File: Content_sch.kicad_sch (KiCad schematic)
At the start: 0 parts

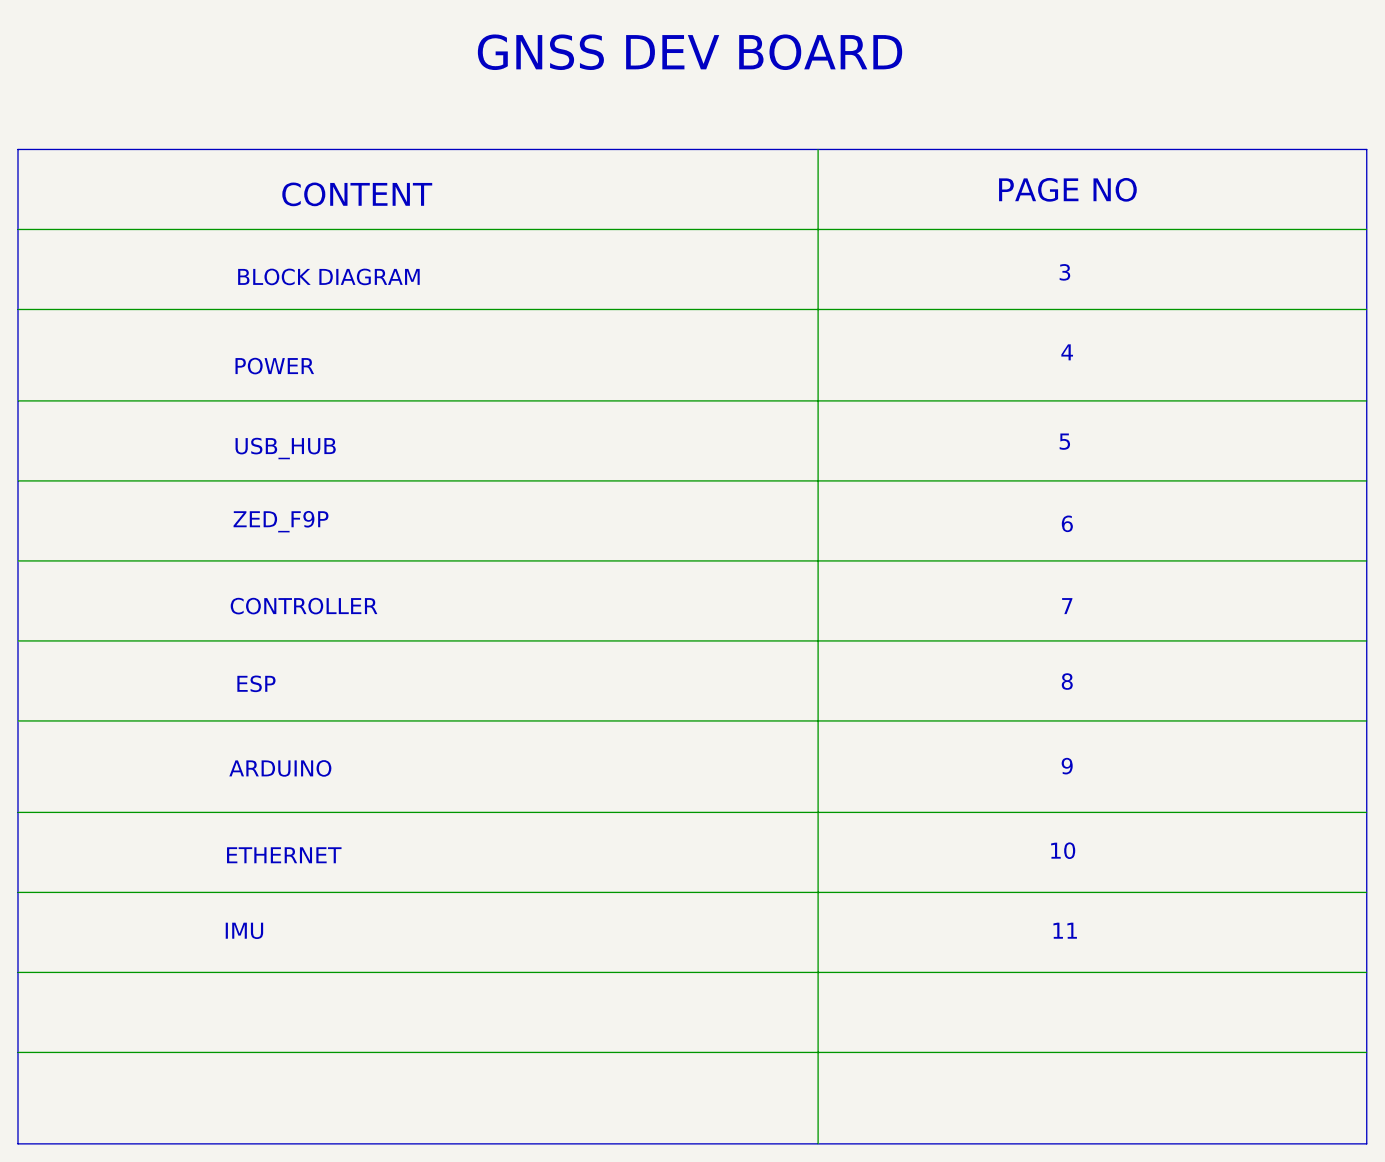
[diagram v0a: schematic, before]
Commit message: changed
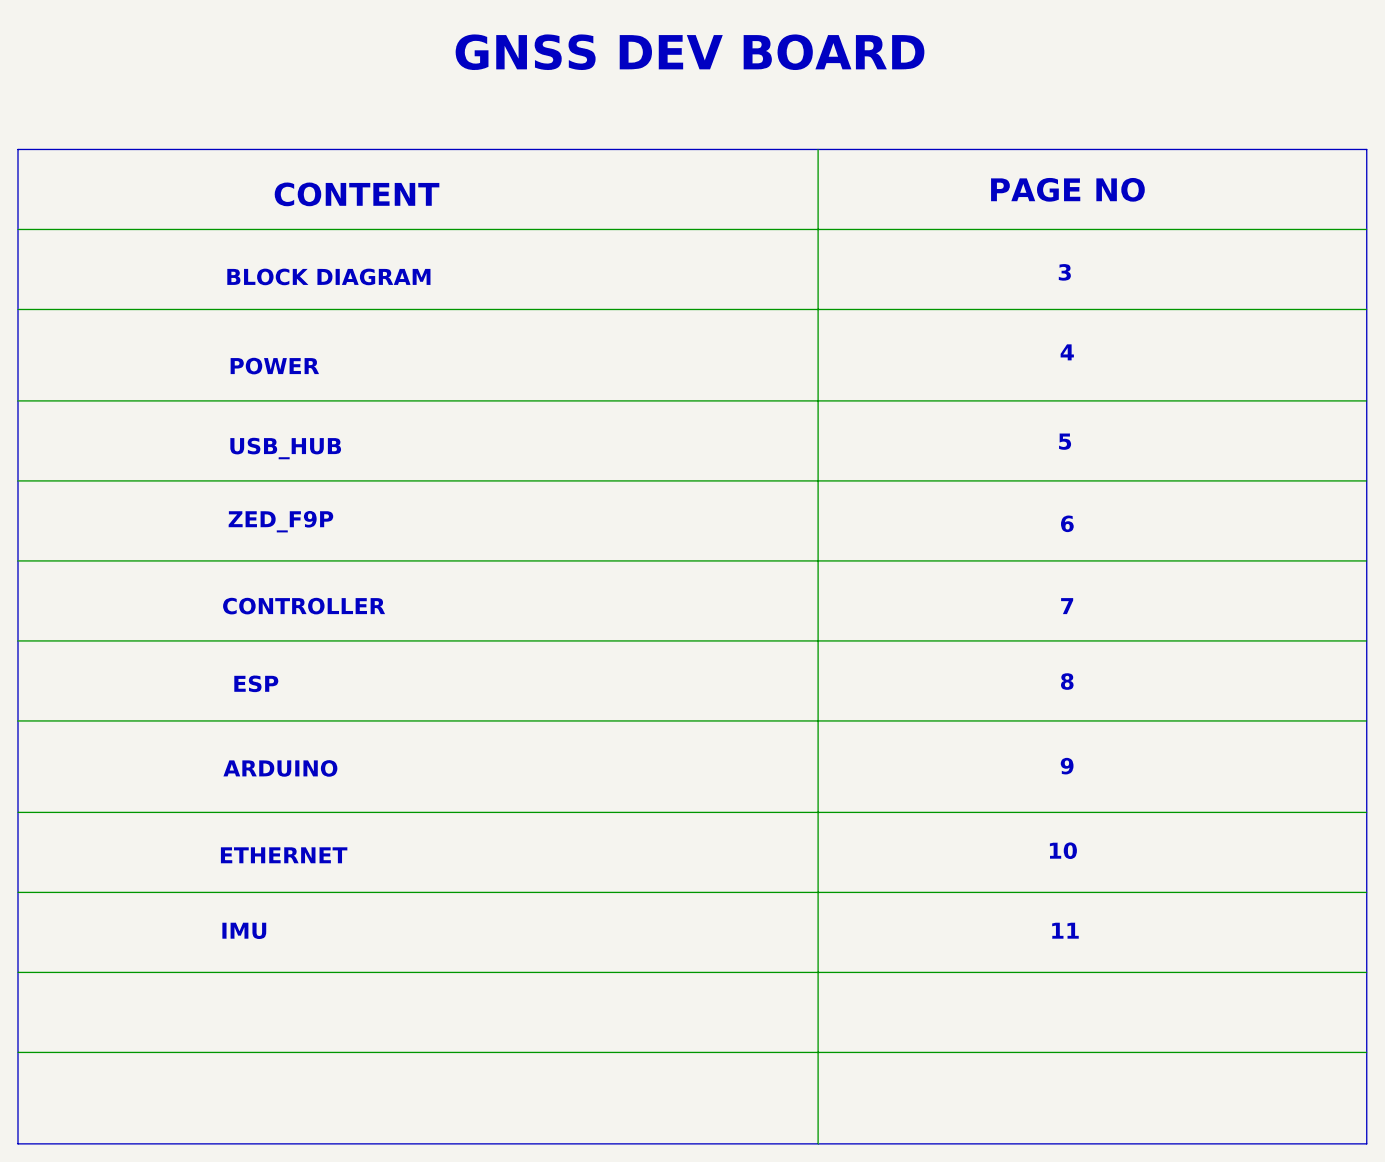
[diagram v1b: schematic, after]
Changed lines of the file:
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@@
 			(font
 				(size 1.778 1.778)
+				(bold yes)
 			)
 		)
@@
 			(font
 				(size 1.778 1.778)
+				(bold yes)
 			)
 		)
@@
 			(font
 				(size 1.778 1.778)
+				(bold yes)
 			)
 		)
@@
 			(font
 				(size 1.778 1.778)
+				(bold yes)
 			)
 		)
@@
 			(font
 				(size 1.778 1.778)
+				(bold yes)
 			)
 		)
@@
 			(font
 				(size 1.778 1.778)
+				(bold yes)
 			)
 		)
@@
 			(font
 				(size 1.778 1.778)
+				(bold yes)
 			)
 		)
@@
 			(font
 				(size 1.778 1.778)
+				(bold yes)
 			)
 		)
@@
 			(font
 				(size 1.778 1.778)
+				(bold yes)
 			)
 		)
@@
 			(font
 				(size 1.778 1.778)
+				(bold yes)
 			)
 		)
@@
 			(font
 				(size 3.81 3.81)
+				(bold yes)
 			)
 		)
@@
 			(font
 				(size 1.778 1.778)
+				(bold yes)
 			)
 		)
@@
 			(font
 				(size 1.778 1.778)
+				(bold yes)
 			)
 		)
@@
 			(font
 				(size 2.54 2.54)
+				(bold yes)
 			)
 		)
@@
 			(font
 				(size 1.778 1.778)
+				(bold yes)
 			)
 		)
@@
 			(font
 				(size 1.778 1.778)
+				(bold yes)
 			)
 		)
@@
 			(font
 				(size 1.778 1.778)
+				(bold yes)
 			)
 		)
@@
 			(font
 				(size 1.778 1.778)
+				(bold yes)
 			)
 		)
@@
 			(font
 				(size 2.54 2.54)
+				(bold yes)
 			)
 		)
@@
 			(font
 				(size 1.778 1.778)
+				(bold yes)
 			)
 		)
@@
 			(font
 				(size 1.778 1.778)
-			)
-		)
+				(bold yes)
+			)
+		)
